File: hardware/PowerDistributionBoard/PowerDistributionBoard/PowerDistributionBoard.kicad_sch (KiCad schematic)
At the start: 17 parts, among them J1 Conn_01x02, Q1 Q_NMOS_GDS, SW1 SW_SPST, U1 LT1641-1

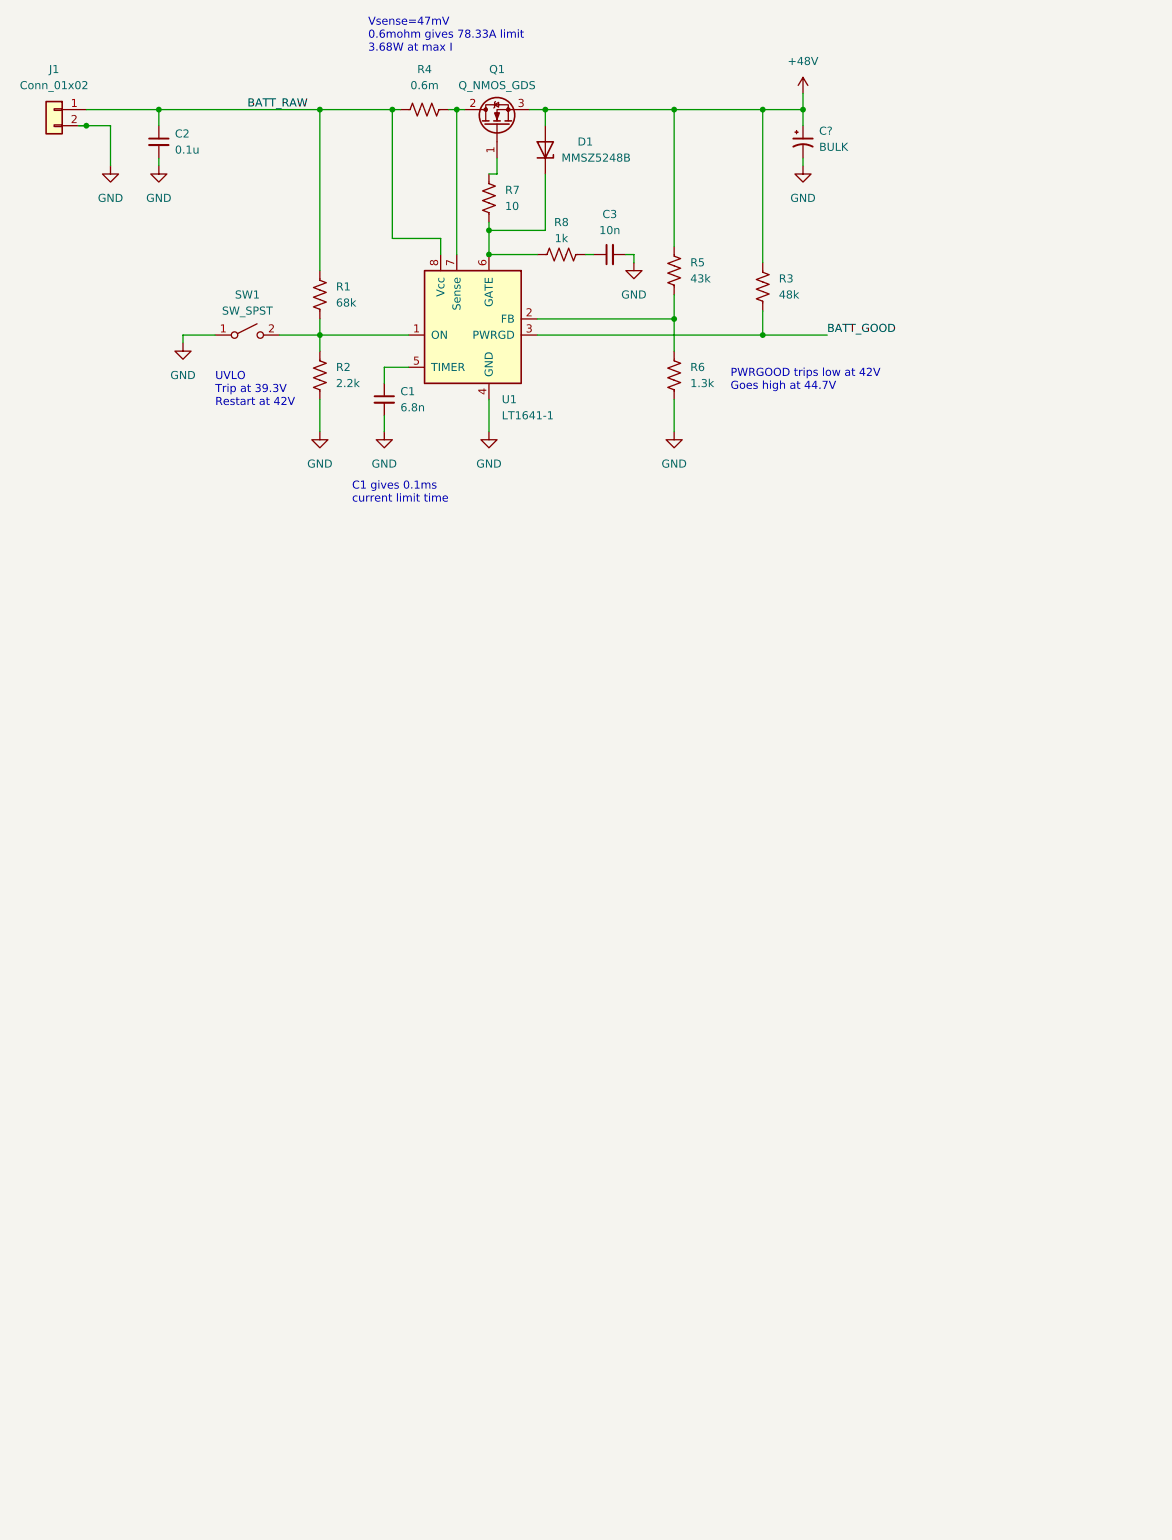
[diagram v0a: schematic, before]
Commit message: Fan Control
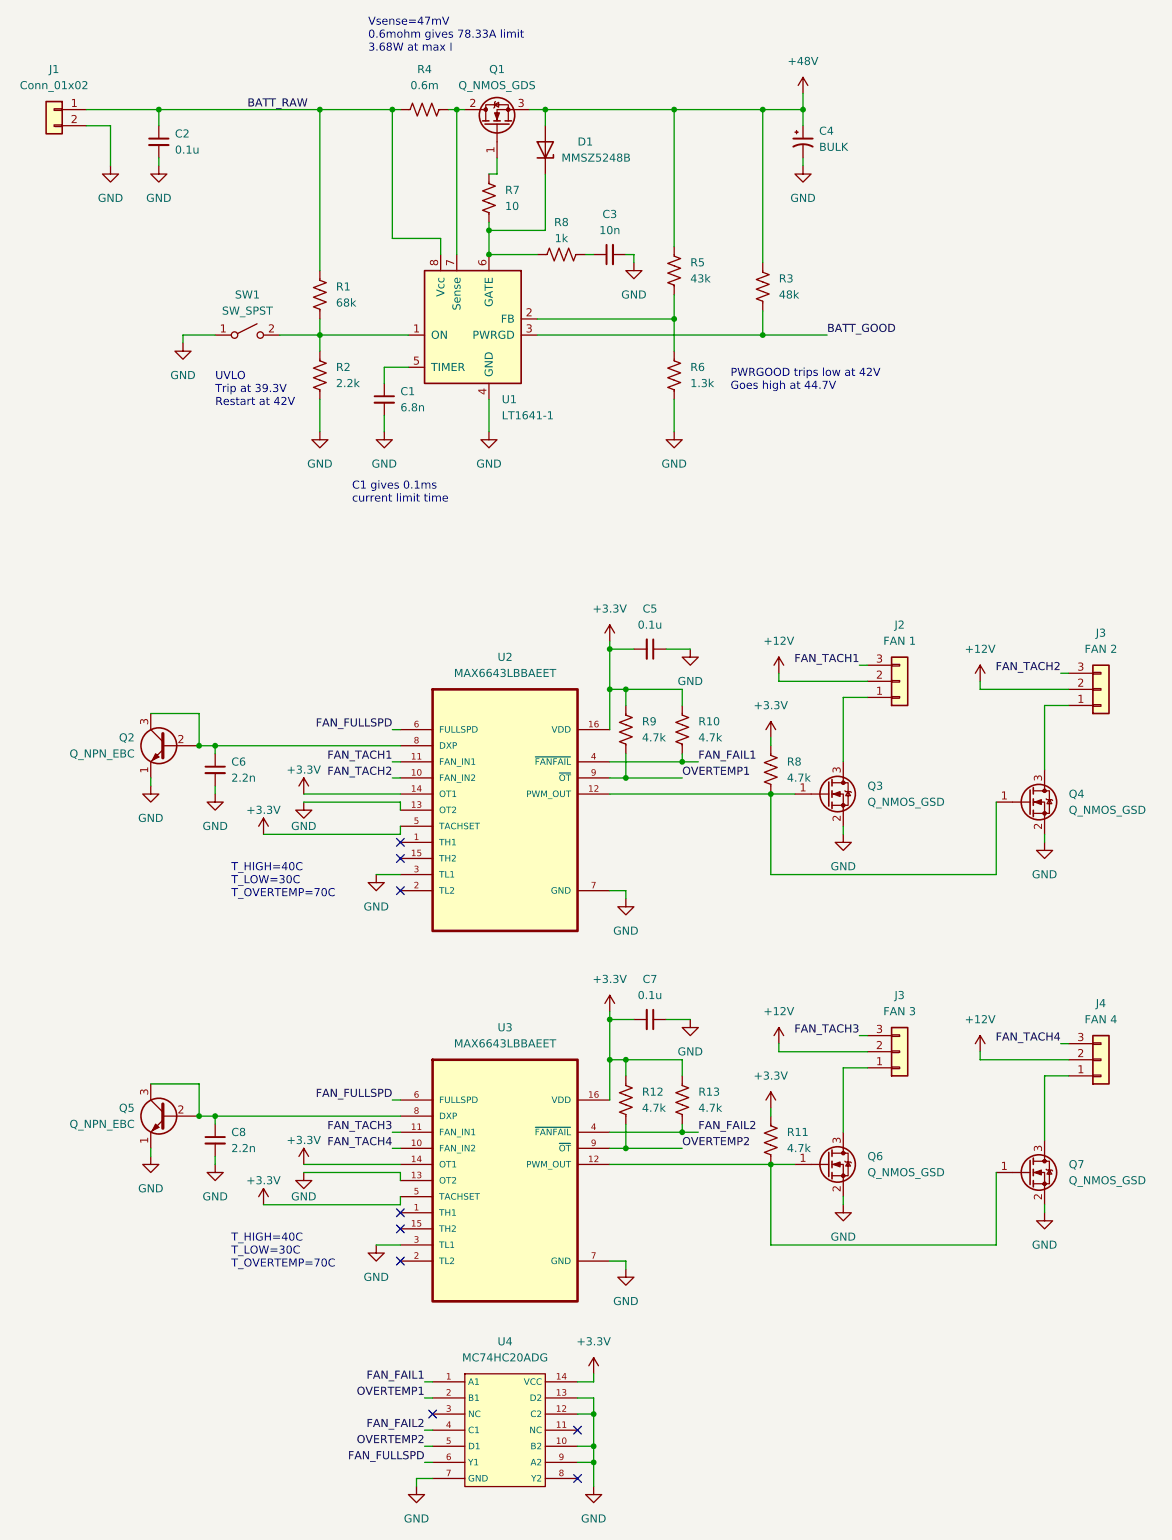
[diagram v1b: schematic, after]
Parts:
- added C5, C7: 0.1u, symbol Device:C_Small
- added C6, C8: 2.2n, symbol Device:C_Small
- added J2: FAN 1, symbol Connector_Generic:Conn_01x03
- added J3: FAN 3, symbol Connector_Generic:Conn_01x03
- added J3: FAN 2, symbol Connector_Generic:Conn_01x03
- added J4: FAN 4, symbol Connector_Generic:Conn_01x03
- added Q2, Q5: Q_NPN_EBC, symbol Device:Q_NPN_EBC
- added Q3, Q4, Q6, Q7: Q_NMOS_GSD, symbol Device:Q_NMOS_GSD
- added R10, R11, R12, R13, R8, R9: 4.7k, symbol Device:R_US
- added U2, U3: MAX6643LBBAEET, SOP63P602X175-16N, symbol PBD_LIB:MAX6643LBBAEET
- added U4: MC74HC20ADG, symbol PBD_LIB:MC74HC20ADG
- gave numbers to parts that had none: 1
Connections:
- net GND: now also C5.1, C6.2, C7.1, C8.2, Q2.1 (E), Q3.2 (S), Q4.2 (S), Q5.1 (E), Q6.2 (S), Q7.2 (S), U2.13 (OT2), U2.3 (TL1), U2.7 (GND), U3.13 (OT2), U3.3 (TL1), U3.7 (GND), U4.10 (B2), U4.12 (C2), U4.13 (D2), U4.7 (GND), U4.9 (A2)
- new net: Q3.1 (G), Q4.1 (G), R8.2, U2.12 (PWM_OUT)
- new net: J2.1 (Pin_1), Q3.3 (D)
- new net: C6.1, Q2.2 (B), Q2.3 (C), U2.8 (DXP)
- new net: C8.1, Q5.2 (B), Q5.3 (C), U3.8 (DXP)
- new net: J3.1 (Pin_1), Q6.3 (D)
- new net: Q6.1 (G), Q7.1 (G), R11.2, U3.12 (PWM_OUT)
- new net: J4.1 (Pin_1), Q7.3 (D)
- new net: J3.1 (Pin_1), Q4.3 (D)
- new net +12V: J2.2 (Pin_2), J3.2 (Pin_2), J3.2 (Pin_2), J4.2 (Pin_2)
- new net +3.3V: C5.2, C7.2, R10.1, R11.1, R12.1, R13.1, R8.1, R9.1, U2.14 (OT1), U2.16 (VDD), U2.5 (TACHSET), U3.14 (OT1), U3.16 (VDD), U3.5 (TACHSET), U4.14 (VCC)
- new net FAN_FAIL1: R10.2, U2.4 (~{FANFAIL}), U4.1 (A1)
- new net FAN_FAIL2: R13.2, U3.4 (~{FANFAIL}), U4.4 (C1)
- new net FAN_FULLSPD: U2.6 (FULLSPD), U3.6 (FULLSPD), U4.6 (Y1)
- new net FAN_TACH1: J2.3 (Pin_3), U2.11 (FAN_IN1)
- new net FAN_TACH2: J3.3 (Pin_3), U2.10 (FAN_IN2)
- new net FAN_TACH3: J3.3 (Pin_3), U3.11 (FAN_IN1)
- new net FAN_TACH4: J4.3 (Pin_3), U3.10 (FAN_IN2)
- new net OVERTEMP1: R9.2, U2.9 (~{OT}), U4.2 (B1)
- new net OVERTEMP2: R12.2, U3.9 (~{OT}), U4.5 (D1)
- no-connect marks 0 -> 9
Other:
- note added: "T_HIGH=40C T_LOW=30C T_OVERTEMP=70C"
